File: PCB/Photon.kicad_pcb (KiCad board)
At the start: 2 copper layers, 21.2 x 74.4 mm, 45 parts, among them J1 USB_C_Receptacle_USB2.0_6P, J2 Conn_01x05_Socket, Q1 IRLML6402, Q2 IRLML6402, SW1 TS-1088-AR02016, U1 STM32G030F6P6TR, U2 TP4056, U3 RT8059GJ5, U4 DW01A, U5 FS8205A, U6 BCR421UW6-7, U7 BCR421UW6-7

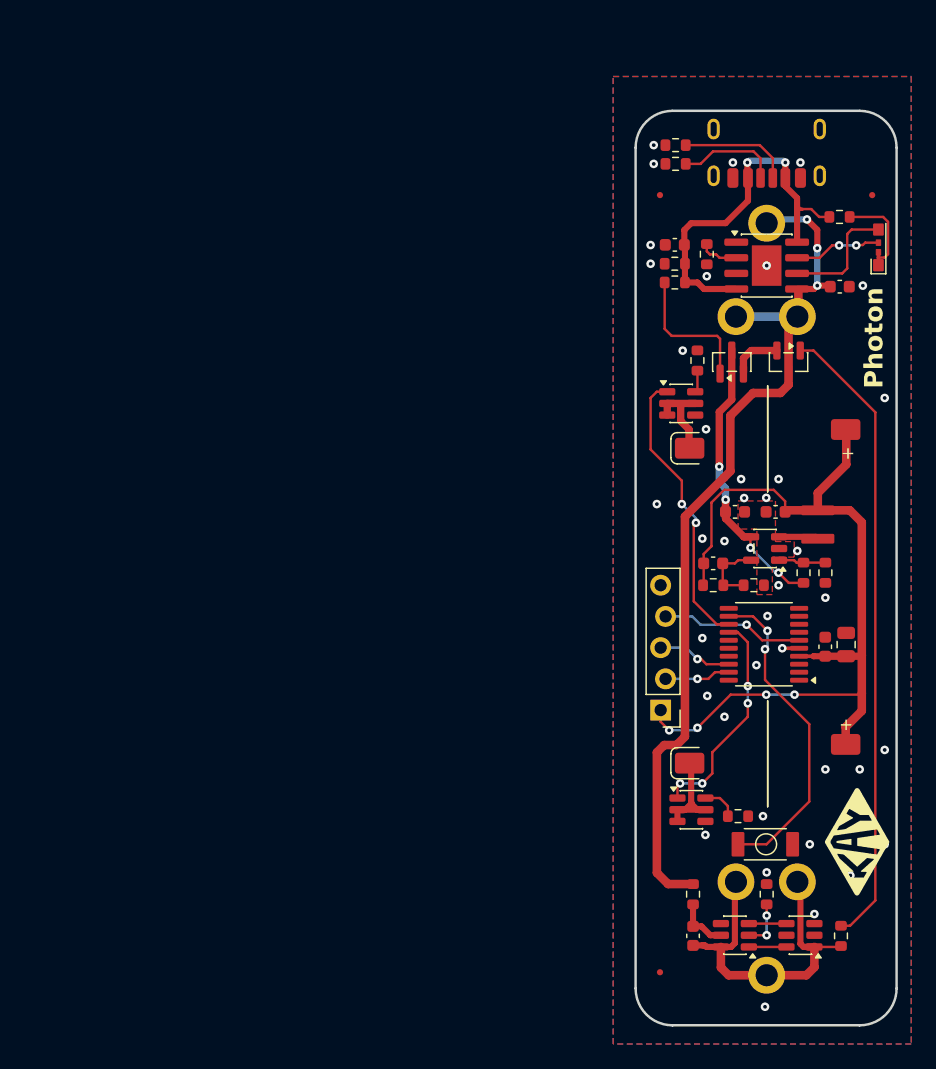
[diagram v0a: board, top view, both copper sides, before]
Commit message: added gerbers
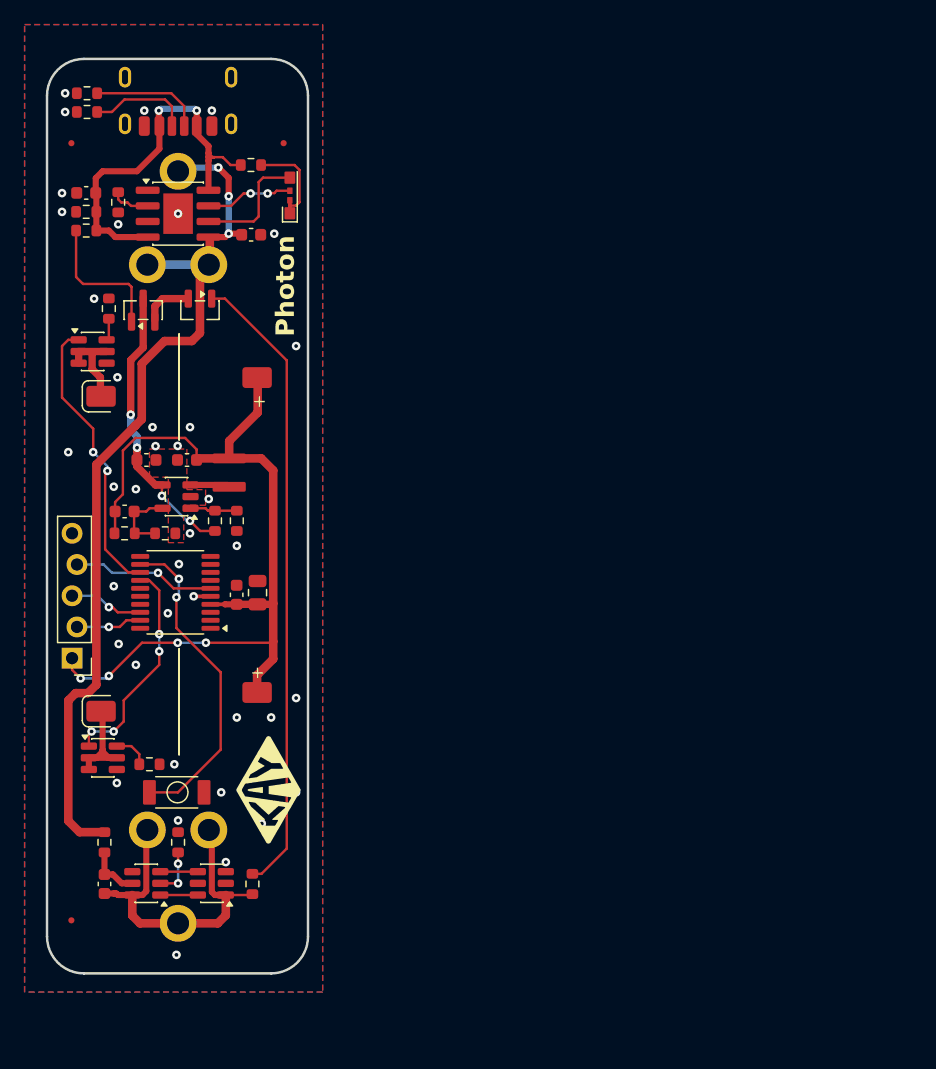
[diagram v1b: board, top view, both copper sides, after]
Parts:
- moved C3 48.1 mm to (42.0, 34.5)
- moved C4 48.1 mm to (46.9, 56.2)
- moved C5 48.1 mm to (55.4, 37.9)
- moved C8 48.1 mm to (43.4, 90.7)
- moved R1 48.1 mm to (42.0, 26.4)
- moved R10 48.1 mm to (48.4, 62.2)
- moved R11 48.1 mm to (43.4, 87.3)
- moved R15 48.1 mm to (47.1, 81.0)
- moved R2 48.1 mm to (42.0, 27.9)
- moved R7 48.1 mm to (42.0, 37.5)
- moved R8 48.1 mm to (42.0, 36.0)
- moved SW1 48.1 mm to (49.4, 83.3)
- moved U5 48.1 mm to (52.2, 90.7)
- moved U6 48.1 mm to (42.5, 47.4)
- moved BT1 48.1 mm to (43.9, 37.3)
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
